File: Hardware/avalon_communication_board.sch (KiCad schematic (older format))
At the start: 21 parts, among them IC1 ENC28J60-I/SO, J1 RJ45_LEDS, P1 B2P-VH, Q1 FMMT597, Q2 BC817, Q3 BC817, Q4 FMMT597, Q5 BC817

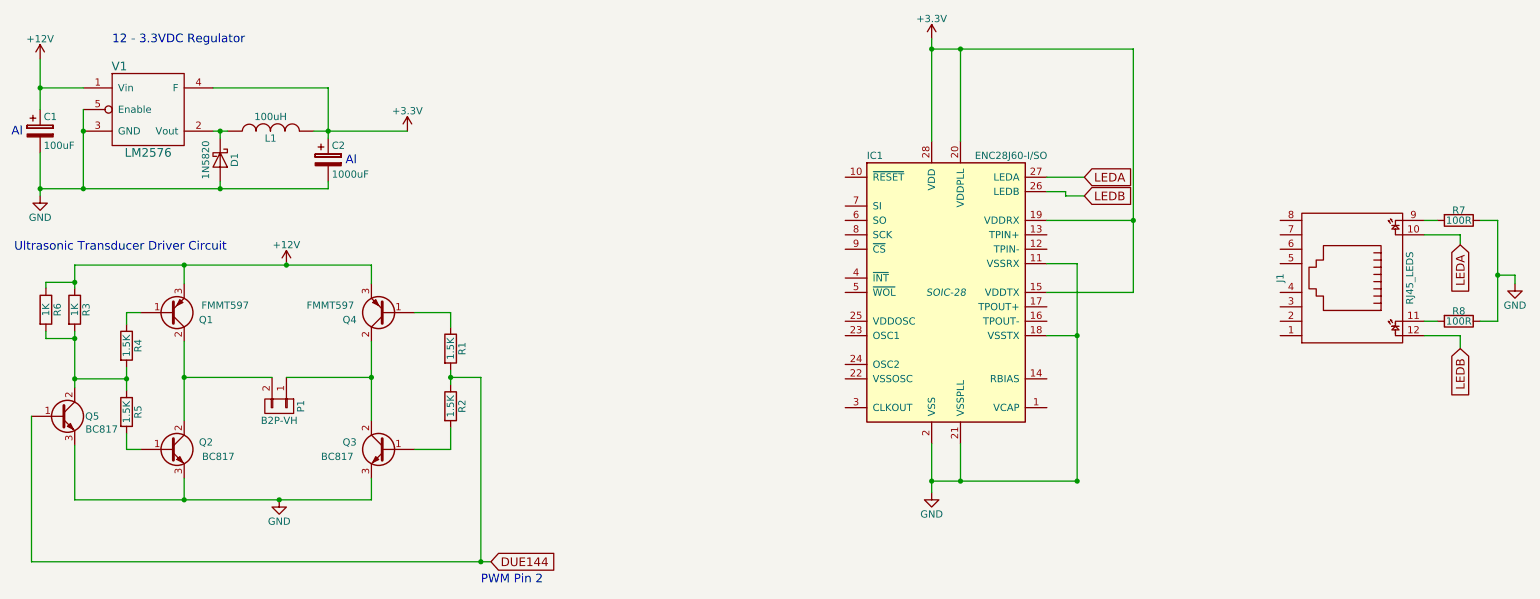
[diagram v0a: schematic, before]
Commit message: -Continued work on the ethernet controller
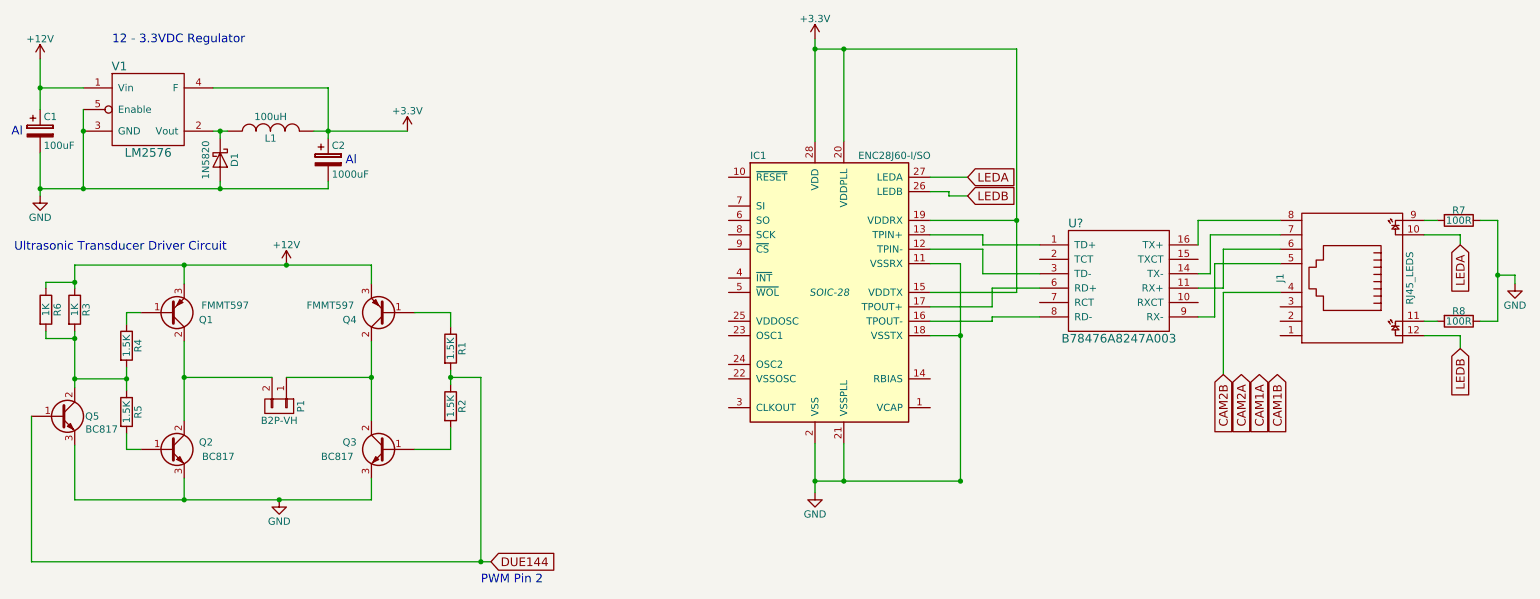
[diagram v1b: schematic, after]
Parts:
- added U?: B78476A8247A003, symbol B78476A8247A003
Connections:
- net at IC1.12 (TPIN-): now also U?.3 (TD-)
- net at IC1.13 (TPIN+): now also U?.1 (TD+)
- net at IC1.16 (TPOUT-): now also U?.8 (RD-)
- net at IC1.17 (TPOUT+): now also U?.6 (RD+)
- net CAM2B: now reaches J1.4
- net at J1.5: now also U?.9 (RX-)
- net at J1.6: now also U?.11 (RX+)
- net at J1.7: now also U?.14 (TX-)
- net at J1.8: now also U?.16 (TX+)
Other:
- moved on the sheet: IC1
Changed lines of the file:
@@
 L ENC28J60-I/SO IC1
 U 1 1 5A903E11
-P 7090 2470
-F 0 "IC1" H 6540 3420 50  0000 L CNN
-F 1 "ENC28J60-I/SO" H 7290 3420 50  0000 L CNN
-F 2 "SOIC-28" H 7090 2470 50  0000 C CIN
-F 3 "" H 7090 2470 50  0000 C CNN
-	1    7090 2470
+P 6280 2470
+F 0 "IC1" H 5730 3420 50  0000 L CNN
+F 1 "ENC28J60-I/SO" H 6480 3420 50  0000 L CNN
+F 2 "SOIC-28" H 6280 2470 50  0000 C CIN
+F 3 "" H 6280 2470 50  0000 C CNN
+	1    6280 2470
 	1    0    0    -1
 $EndComp
@@
 L +3.3V #PWR6
 U 1 1 5A908CDC
-P 6990 710
-F 0 "#PWR6" H 6990 560 50  0001 C CNN
-F 1 "+3.3V" H 6990 850 50  0000 C CNN
-F 2 "" H 6990 710 50  0000 C CNN
-F 3 "" H 6990 710 50  0000 C CNN
-	1    6990 710
+P 6180 710
+F 0 "#PWR6" H 6180 560 50  0001 C CNN
+F 1 "+3.3V" H 6180 850 50  0000 C CNN
+F 2 "" H 6180 710 50  0000 C CNN
+F 3 "" H 6180 710 50  0000 C CNN
+	1    6180 710
 	1    0    0    -1
 $EndComp
@@
 L GND #PWR7
 U 1 1 5A90B1AB
-P 6990 3860
-F 0 "#PWR7" H 6990 3610 50  0001 C CNN
-F 1 "GND" H 6990 3710 50  0000 C CNN
-F 2 "" H 6990 3860 50  0000 C CNN
-F 3 "" H 6990 3860 50  0000 C CNN
-	1    6990 3860
-	1    0    0    -1
-$EndComp
-Text GLabel 8050 1670 2    60   Input ~ 0
+P 6180 3860
+F 0 "#PWR7" H 6180 3610 50  0001 C CNN
+F 1 "GND" H 6180 3710 50  0000 C CNN
+F 2 "" H 6180 3860 50  0000 C CNN
+F 3 "" H 6180 3860 50  0000 C CNN
+	1    6180 3860
+	1    0    0    -1
+$EndComp
+Text GLabel 7240 1670 2    60   Input ~ 0
 LEDA
-Text GLabel 8050 1800 2    60   Input ~ 0
+Text GLabel 7240 1800 2    60   Input ~ 0
 LEDB
 $Comp
@@
 	10660 2070 10660 2140
 Wire Wire Line
-	6990 780  8390 780
-Wire Wire Line
-	7790 1670 8050 1670
-Wire Wire Line
-	7790 1770 7920 1770
-Wire Wire Line
-	7920 1770 7920 1800
-Wire Wire Line
-	7920 1800 8050 1800
-Wire Wire Line
-	7790 1970 8390 1970
-Wire Wire Line
-	8390 780  8390 2470
-Wire Wire Line
-	6990 710  6990 1420
-Connection ~ 6990 780
-Wire Wire Line
-	7190 1420 7190 780
-Connection ~ 7190 780
-Wire Wire Line
-	8390 2470 7790 2470
-Connection ~ 8390 1970
-Wire Wire Line
-	6990 3520 6990 3860
-Wire Wire Line
-	7190 3520 7190 3780
-Wire Wire Line
-	8000 3780 6990 3780
-Connection ~ 6990 3780
-Wire Wire Line
-	7790 2270 8000 2270
-Wire Wire Line
-	8000 2270 8000 3780
-Wire Wire Line
-	8000 2770 7790 2770
-Connection ~ 8000 2770
+	6180 780  7580 780
+Wire Wire Line
+	6980 1670 7240 1670
+Wire Wire Line
+	6980 1770 7110 1770
+Wire Wire Line
+	7110 1770 7110 1800
+Wire Wire Line
+	7110 1800 7240 1800
+Wire Wire Line
+	6980 1970 7580 1970
+Wire Wire Line
+	7580 780  7580 2470
+Wire Wire Line
+	6180 710  6180 1420
+Connection ~ 6180 780
+Wire Wire Line
+	6380 1420 6380 780
+Connection ~ 6380 780
+Wire Wire Line
+	7580 2470 6980 2470
+Connection ~ 7580 1970
+Wire Wire Line
+	6180 3520 6180 3860
+Wire Wire Line
+	6380 3520 6380 3780
+Wire Wire Line
+	7190 3780 6180 3780
+Connection ~ 6180 3780
+Wire Wire Line
+	6980 2270 7190 2270
+Wire Wire Line
+	7190 2270 7190 3780
+Wire Wire Line
+	7190 2770 6980 2770
+Connection ~ 7190 2770
+Connection ~ 6380 3780
 Connection ~ 7190 3780
-Connection ~ 8000 3780
+$Comp
+L B78476A8247A003 U?
+U 1 1 5A907D1C
+P 8290 2290
+F 0 "U?" H 7990 2590 60  0000 C CNN
+F 1 "B78476A8247A003" H 8290 1790 60  0000 C CNN
+F 2 "" H 8290 2290 60  0001 C CNN
+F 3 "" H 8290 2290 60  0001 C CNN
+	1    8290 2290
+	1    0    0    -1
+$EndComp
+Wire Wire Line
+	8840 1970 9410 1970
+Wire Wire Line
+	8925 2070 9410 2070
+Wire Wire Line
+	8925 2070 8925 2340
+Wire Wire Line
+	8840 2440 9015 2440
+Wire Wire Line
+	8955 2270 9410 2270
+Wire Wire Line
+	8925 2340 8840 2340
+Wire Wire Line
+	6980 2070 7345 2070
+Wire Wire Line
+	7345 2070 7345 2140
+Wire Wire Line
+	7345 2140 7740 2140
+Wire Wire Line
+	7345 2340 7740 2340
+Wire Wire Line
+	7345 2340 7345 2170
+Wire Wire Line
+	7345 2170 6980 2170
+Wire Wire Line
+	6980 2570 7410 2570
+Wire Wire Line
+	7410 2570 7410 2440
+Wire Wire Line
+	7410 2440 7740 2440
+Wire Wire Line
+	6980 2670 7410 2670
+Wire Wire Line
+	7410 2670 7410 2640
+Wire Wire Line
+	7410 2640 7740 2640
+Text GLabel 9265 3040 3    60   Input ~ 0
+CAM1A
+Text GLabel 9390 3040 3    60   Input ~ 0
+CAM1B
+Text GLabel 9140 3040 3    60   Input ~ 0
+CAM2A
+Text GLabel 9015 3040 3    60   Input ~ 0
+CAM2B
+Wire Wire Line
+	8955 2640 8840 2640
+Wire Wire Line
+	8955 2270 8955 2640
+Wire Wire Line
+	9015 2470 9015 3040
+Wire Wire Line
+	9015 2440 9015 2170
+Wire Wire Line
+	9015 2170 9410 2170
+Wire Wire Line
+	9015 2470 9410 2470
+Wire Wire Line
+	8840 1970 8840 2140
 $EndSCHEMATC
